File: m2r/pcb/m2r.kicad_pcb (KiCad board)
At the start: 2 copper layers, 50 x 75 mm, 118 parts, among them IC1 ADP3338, IC10 STM32F303C, IC11 ADP3333, IC2 ADP3335, IC3 ADuM1201, IC4 ADuM1201, IC5 ADuM1201, IC6 MTX2, IC7 ADL5324, IC8 MAX-7Q, IC9 ALM-2712, P1 CONN_2, P2 CONN_2, P3 CONN_4, P4 CONN_4, P5 CONN_4, P6 SWD, P7 SMA, P8 CONN_2, X10 8M, X11 M3 MOUNT, X12 M3 MOUNT, X13 M3 MOUNT, X14 M3 MOUNT

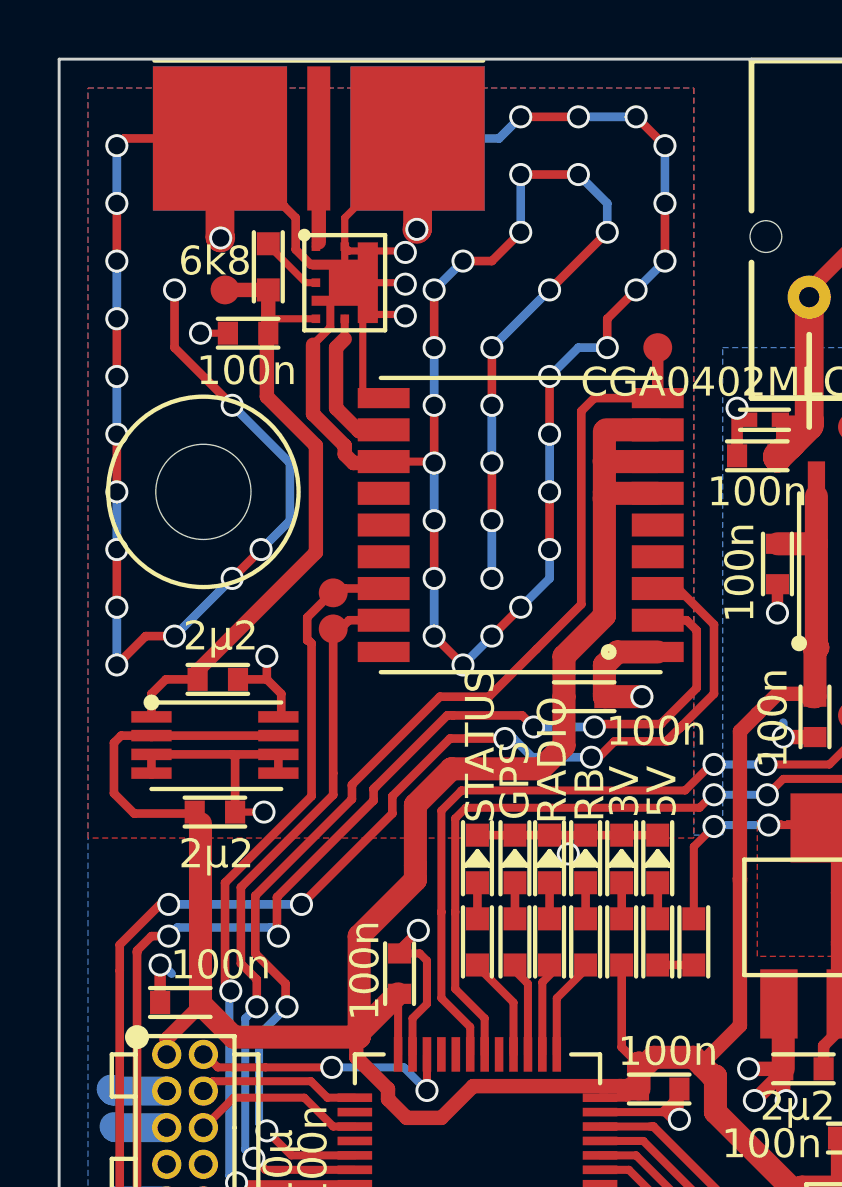
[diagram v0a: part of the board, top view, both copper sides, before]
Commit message: done pls
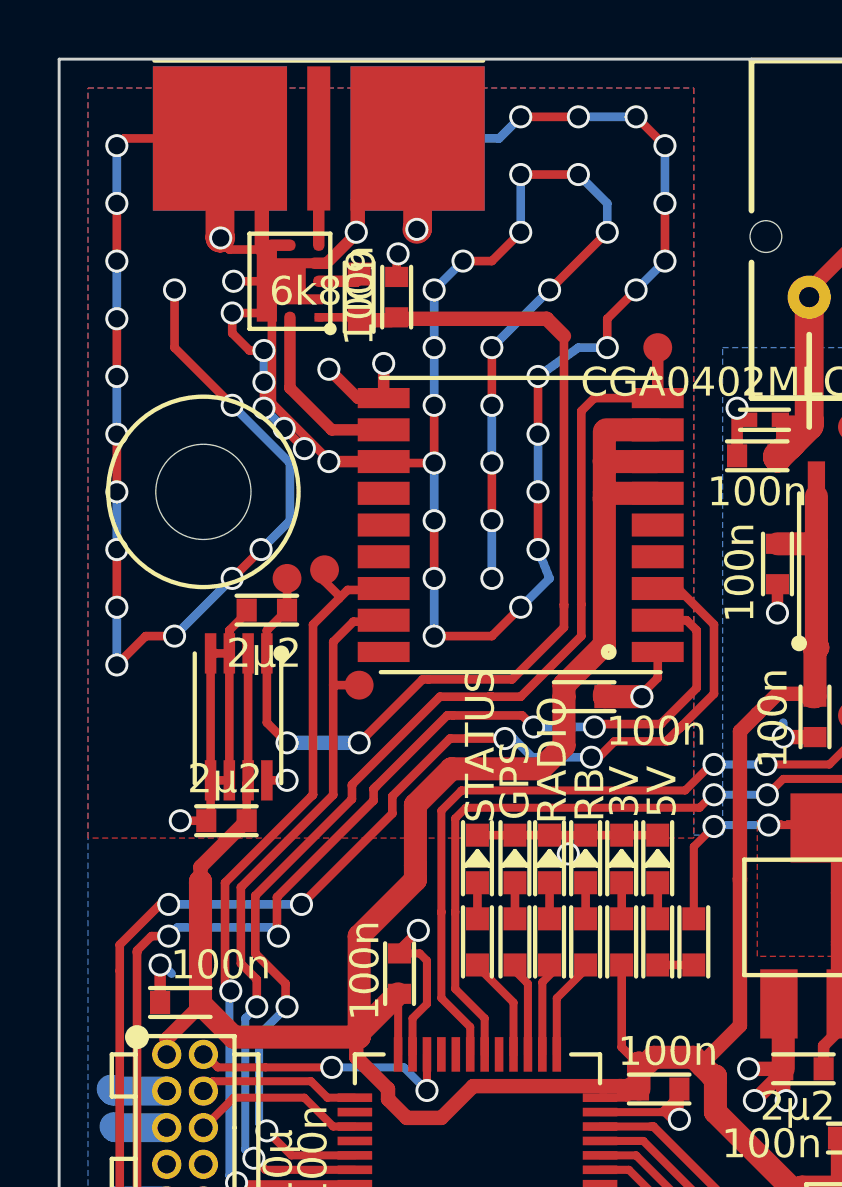
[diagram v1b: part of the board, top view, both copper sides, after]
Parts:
- moved TP18 10.2 mm to (123.9, 77.0)
- moved IC11 4.57 mm to (123.2, 79.6), turned to 270 degrees
- moved C31 4.48 mm to (127.7, 68.0), turned to 90 degrees
- moved C32 3.92 mm to (123.9, 78.1), turned to 180 degrees
- moved R6 3.32 mm to (126.4, 68.0)
- moved IC9 2.58 mm to (125.2, 65.5), turned to 270 degrees
- moved TP20 2.15 mm to (126.4, 80.7)
- moved C33 1.82 mm to (122.5, 85.4), turned to 180 degrees
- moved TP21 0.85 mm to (125.2, 76.7)
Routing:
- net Net-(C31-Pad1): track 21.9 -> 37.2 mm, vias 0 -> 2
- net GND: track 422.1 -> 432.5 mm, vias 150 -> 156
- net +3.3V: track 205.7 -> 201.1 mm
- net Net-(ANT1-Pad1): track 7.57 -> 4.19 mm
- net Net-(IC8-Pad11): track 5.40 -> 6.30 mm
- net GPS_SDA: track 28.4 -> 29.3 mm
- net GPS_RESET: track 39.9 -> 40.6 mm
- net Net-(IC9-Pad11): track 2.27 -> 1.62 mm
- net GPS_SCL: track 25.7 -> 26.4 mm
